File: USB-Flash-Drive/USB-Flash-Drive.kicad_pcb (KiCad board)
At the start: 2 copper layers, 19.4 x 49.1 mm, 37 parts, among them J1 USB_A, J2 Conn_01x03_Pin, U1 RP2040, U2 W25Q128JVS, U3 AMS1117, U4 W25N01GVZEIG, Y2 ABM8-272-T3

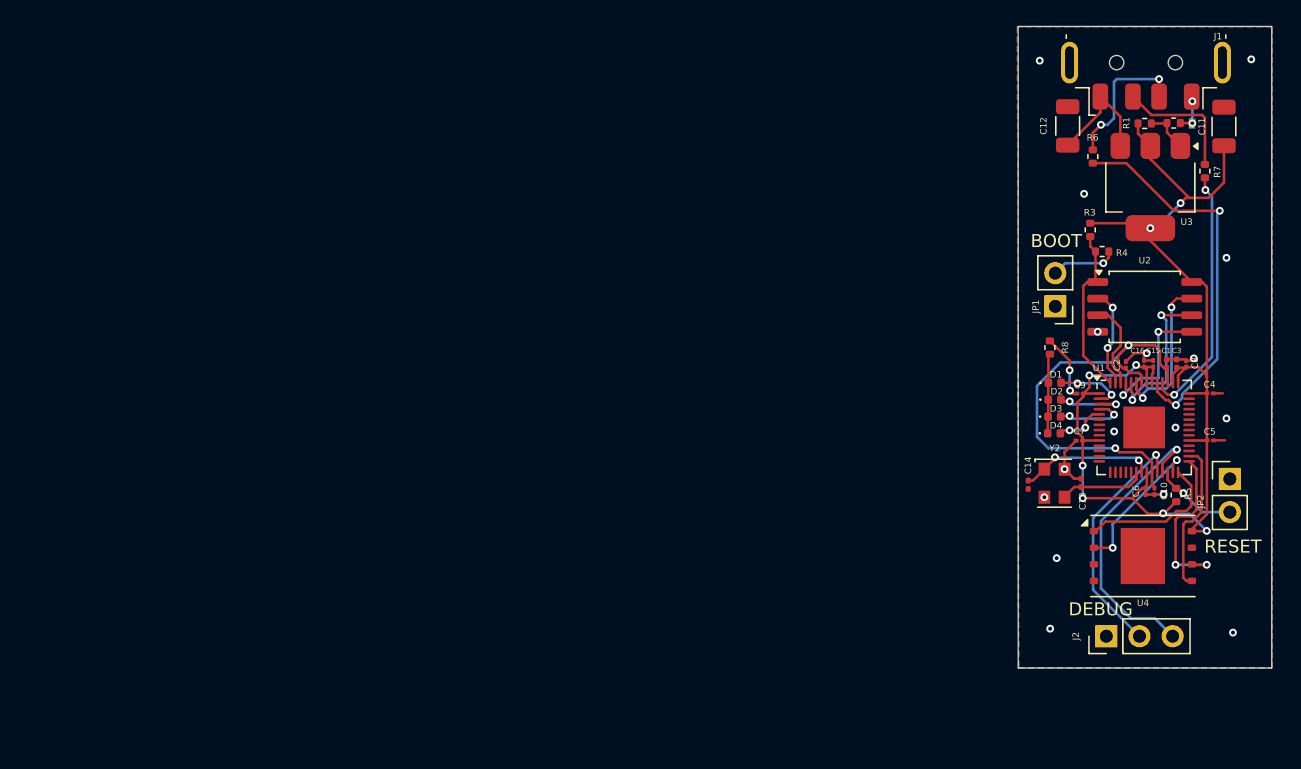
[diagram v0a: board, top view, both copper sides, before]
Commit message: USB-Thumb-Drive V2
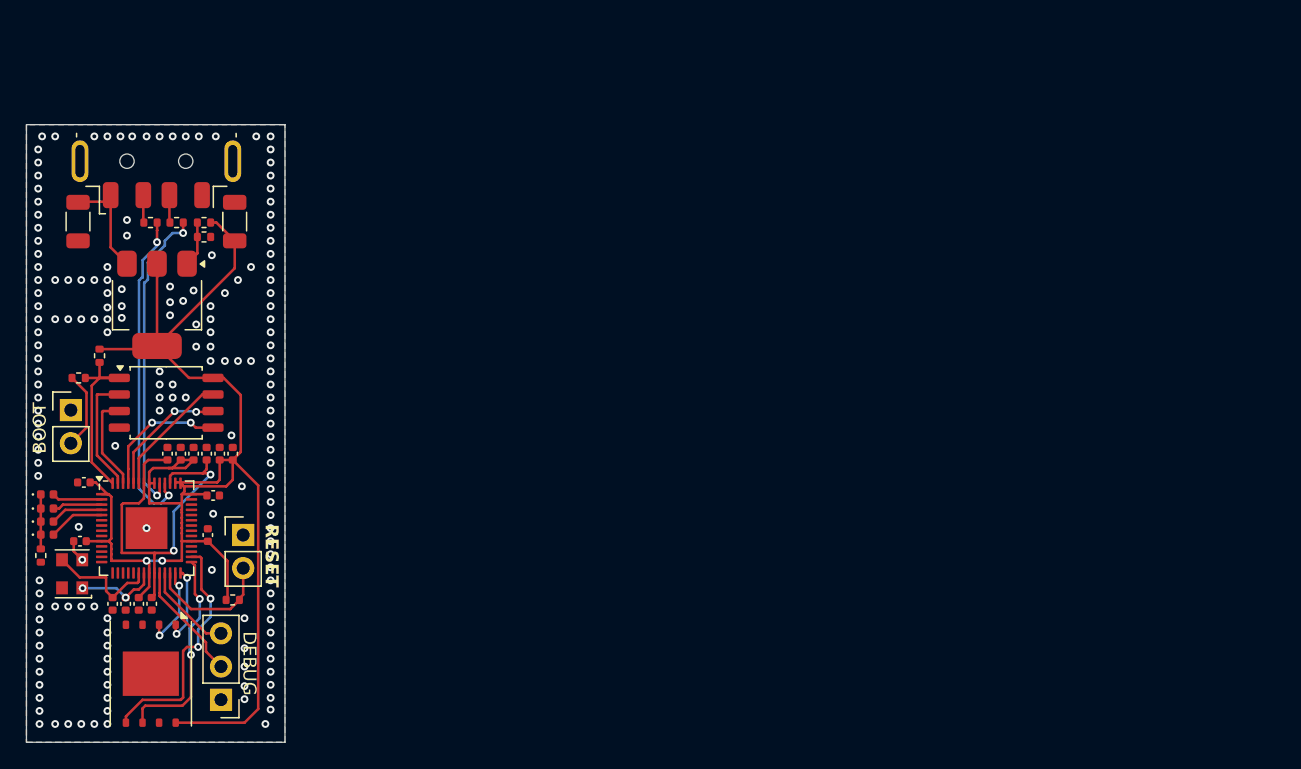
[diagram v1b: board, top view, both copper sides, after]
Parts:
- added G***: LOGO, LOGO, B.Cu at (112.3, 137.9)
- C1, C13, C14, C3: footprint Capacitor_SMD:C_0201_0603Metric -> Capacitor_SMD:C_0402_1005Metric
- C10, C15, C16, C2, C4, C5, C6, C7, C8, C9: footprint Capacitor_SMD:C_01005_0402Metric -> Capacitor_SMD:C_0402_1005Metric
- U2: footprint Package_SO:SOIC-8_5.23x5.23mm_P1.27mm -> Package_SO:SOIC-8_5.3x5.3mm_P1.27mm
- moved C8 82.3 mm to (107.4, 143.8), turned to 90 degrees
- moved C16 81.7 mm to (103.2, 134.5), turned to 0 degrees
- moved R7 80.8 mm to (108.3, 114.6), turned to 0 degrees
- moved R4 79.0 mm to (102.8, 126.5), turned to 0 degrees
- moved R8 78.9 mm to (99.9, 140.1), turned to 90 degrees
- moved C5 77.9 mm to (111.6, 132.3), turned to -90 degrees
- moved D1 77.6 mm to (100.4, 135.4)
- moved D2 77.6 mm to (100.4, 136.5)
- moved D3 77.6 mm to (100.4, 137.5)
- moved D4 77.5 mm to (100.4, 138.5)
- moved C9 77.4 mm to (102.9, 139.0)
- moved C10 77.3 mm to (108.4, 143.8)
- moved U1 76.8 mm to (108.0, 138.0)
- moved C4 76.7 mm to (113.1, 135.5)
- moved U3 76.6 mm to (108.8, 120.9)
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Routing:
- net IOVDD: track 92.2 -> 120.2 mm, vias 8 -> 2
- net GND: track 20.6 -> 1.70 mm, vias 20 -> 172
- net Net-(J2-Pin_3): track 22.5 -> 7.07 mm, vias 1 -> 0
- net Net-(J2-Pin_2): track 18.7 -> 9.11 mm, vias 1 -> 0
- net USBD+: track 11.0 -> 2.12 mm, vias 2 -> 0
- net USBD-: track 9.76 -> 2.12 mm
- net /SPI_COPI: track 11.5 -> 18.6 mm, vias 0 -> 2
- net Net-(U1-USB_DP): track 30.1 -> 24.1 mm
- net Net-(U1-USB_DM): track 19.6 -> 25.0 mm
- net /SPI_CS: track 11.1 -> 6.01 mm, vias 0 -> 2
- net /SPI_CIPO: track 11.1 -> 6.45 mm
- net /XOUT: track 10.3 -> 6.32 mm
- net DVDD: track 33.7 -> 29.9 mm
- net /RESET: track 6.36 -> 9.98 mm, vias 1 -> 0
- net /SPI_CLK: track 13.0 -> 16.1 mm
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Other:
- board size 19.4 x 49.1 mm -> 19.8 x 47.3 mm
- board text added: "128MB USB Flash Drive"
- board text removed: "128MB Thumb Drive v1.0.0"
- board text removed: "Designed by: Cooper Werner"
